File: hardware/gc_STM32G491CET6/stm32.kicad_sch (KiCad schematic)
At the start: 22 parts, among them J7 Conn_02x07_Odd_Even, U301 STM32G491CET6, Y301 16MHz

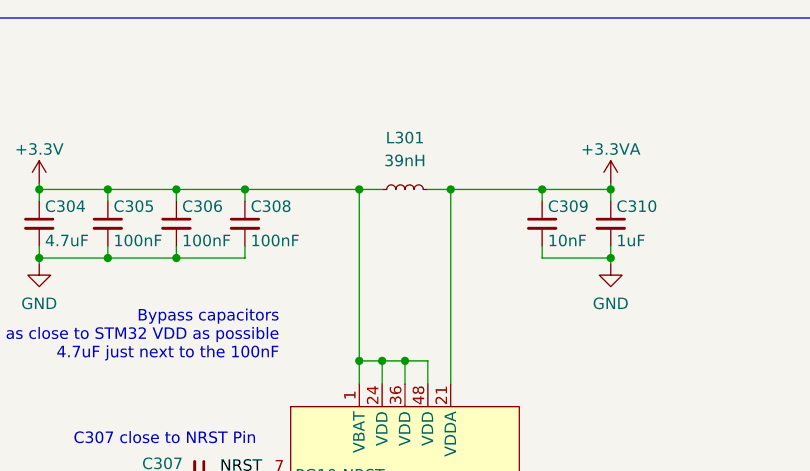
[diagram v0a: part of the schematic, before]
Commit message: silkscreen
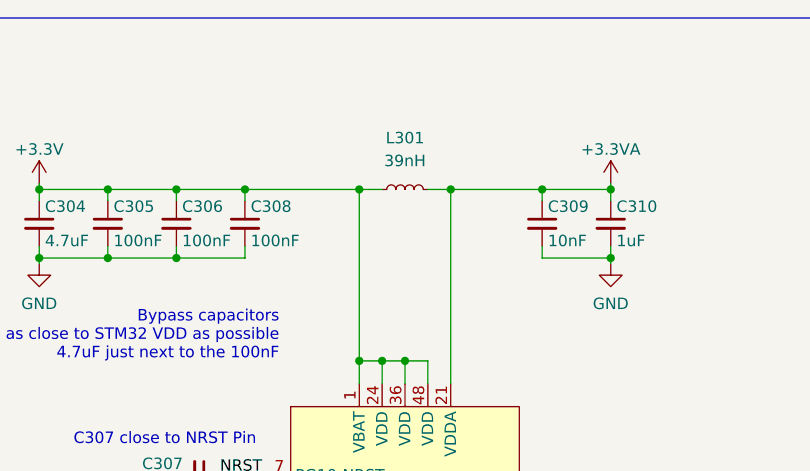
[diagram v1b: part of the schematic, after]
